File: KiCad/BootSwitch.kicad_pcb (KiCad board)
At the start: 2 copper layers, 11 parts, among them J1 JCOM1, J2 Molex 8981-P04, SW1 Case Switch, U1 ATtiny85-20PU, U2 MAX232

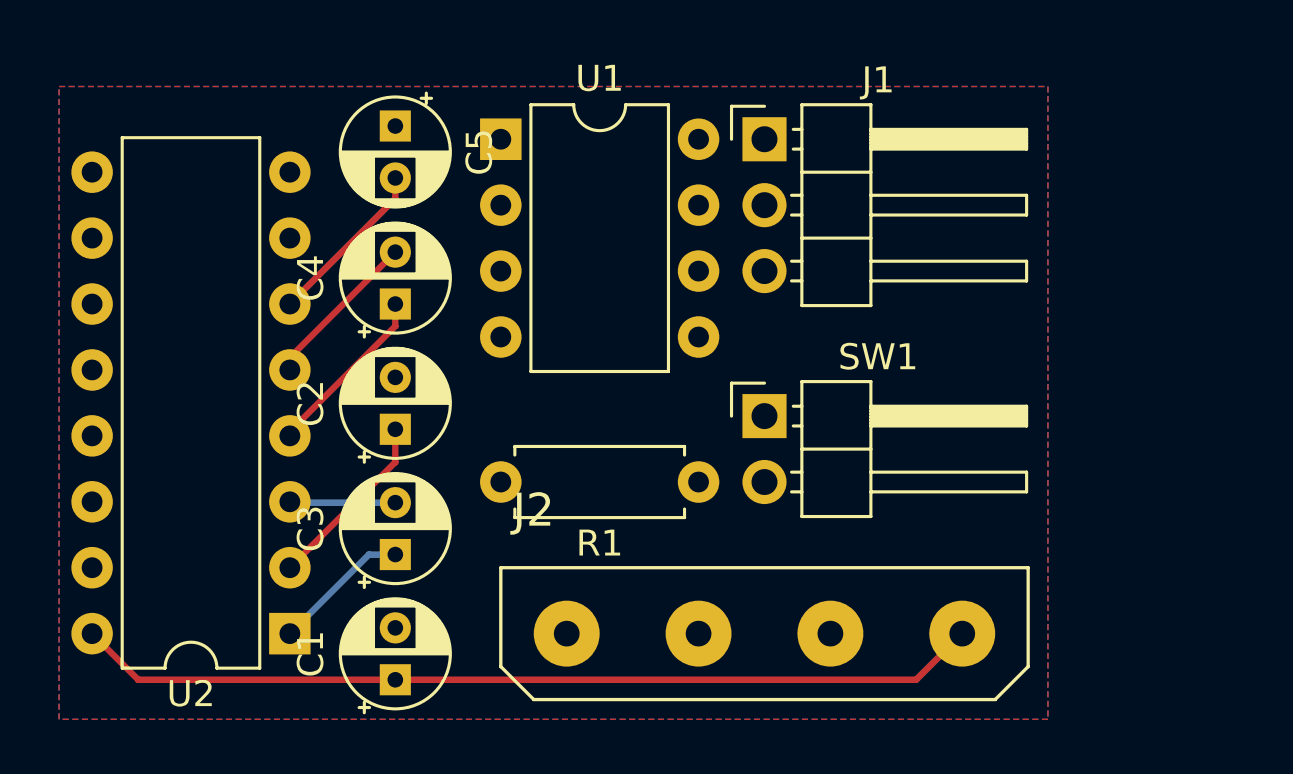
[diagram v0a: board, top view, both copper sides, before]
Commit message: Revise PCB for production
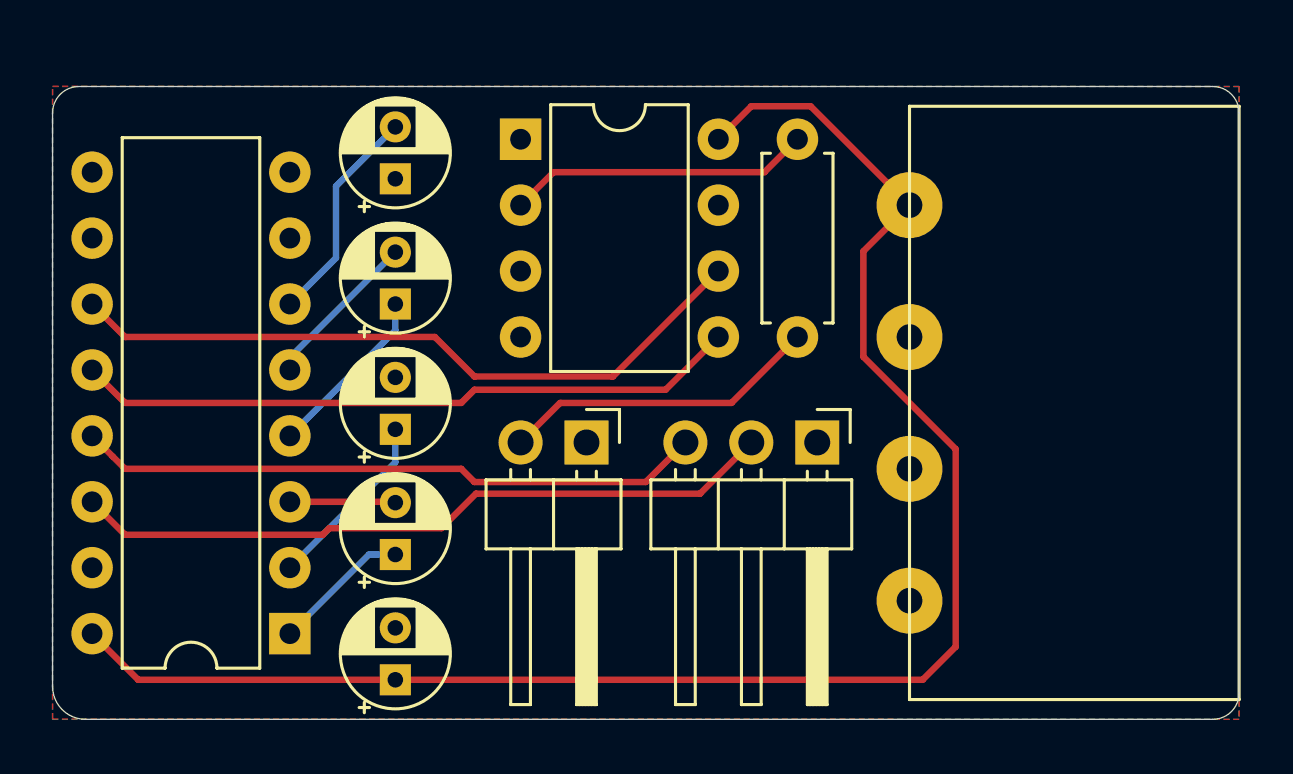
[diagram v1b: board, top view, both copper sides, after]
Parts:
- J2: footprint xess:xess-MOLEX-8981-04P -> BootSwitch:MOLEX_8981_4P_Horizontal
- moved J1 11.9 mm to (179.8, 49.8), turned to 270 degrees
- moved SW1 6.93 mm to (170.9, 49.8), turned to 270 degrees
- moved R1 6.76 mm to (179.1, 45.7), turned to 90 degrees
- moved J2 5.73 mm to (183.4, 55.9), turned to 90 degrees
- moved C5 2.03 mm to (163.6, 39.6), turned to 90 degrees
- moved U1 0.76 mm to (168.4, 38.1)
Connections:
- J1 pad 1: Net-(J1-Pad1) -> Earth
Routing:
- net 5v: track 35.0 -> 63.2 mm
- net Net-(J1-Pad2): track 0.00 -> 27.4 mm
- net Net-(U1-Pad6): track 0.00 -> 27.0 mm
- net Net-(U1-Pad5): track 0.00 -> 25.7 mm
- net Net-(J1-Pad3): track 0.00 -> 24.2 mm
- net Net-(R1-Pad1): track 0.00 -> 12.4 mm
- net Net-(R1-Pad2): track 0.00 -> 11.7 mm
- net Net-(C5-Pad2): track 6.54 -> 8.51 mm
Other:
- board outline added: 45.7 x 24.4 mm
